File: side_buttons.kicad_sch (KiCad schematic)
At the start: 1 part, among them J4 Conn_01x08

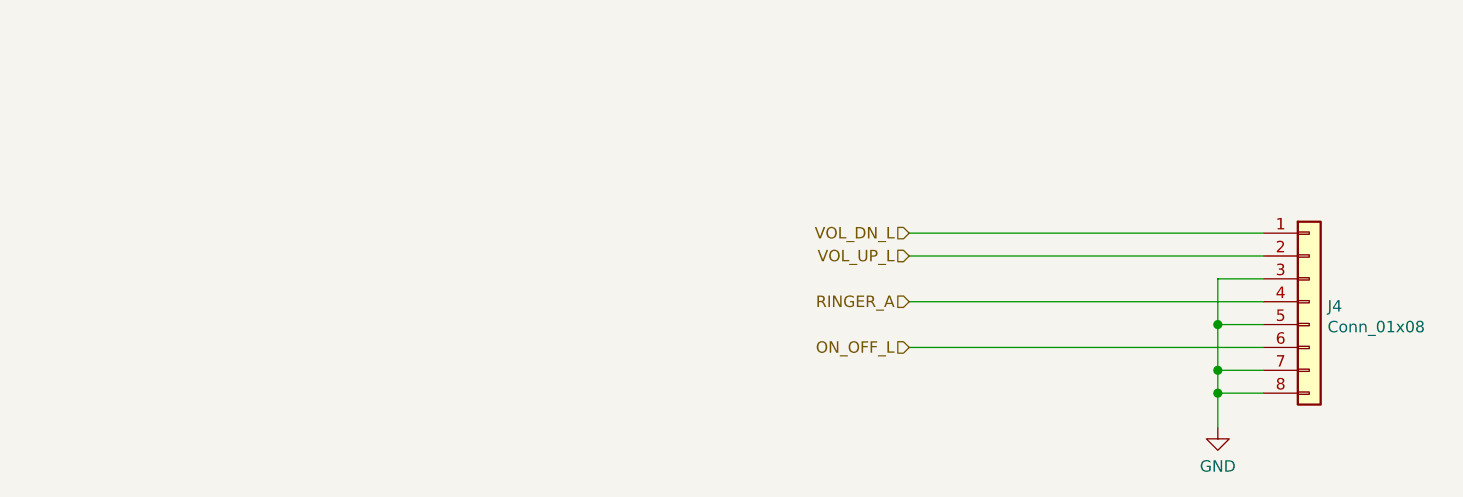
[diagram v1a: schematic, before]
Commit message: Final touches on Radxa CM3 version of the board
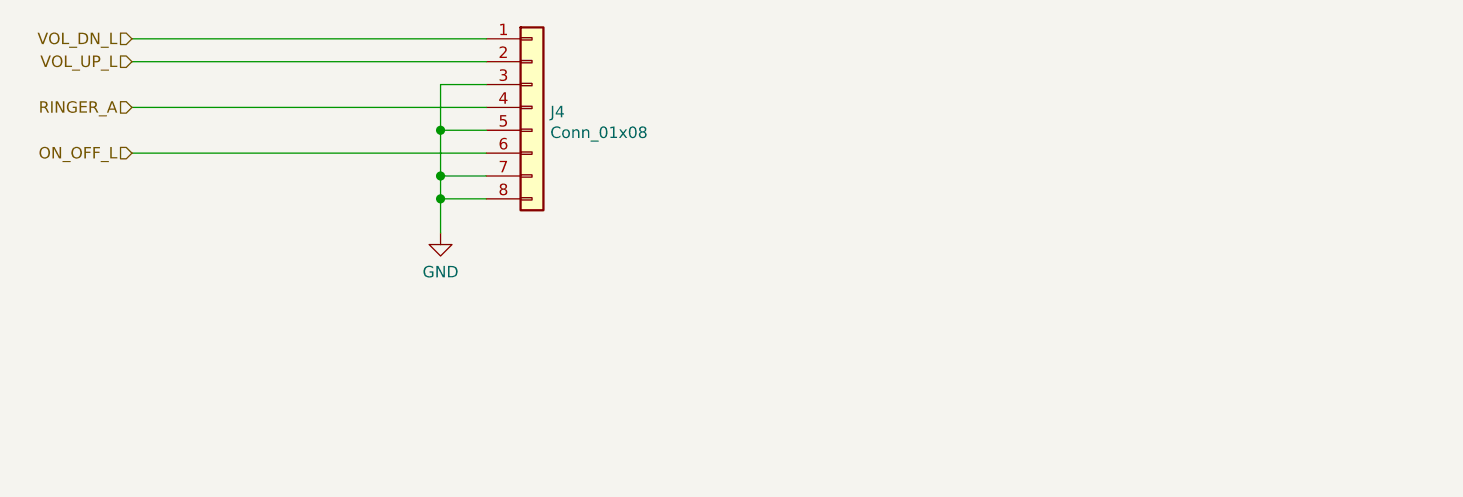
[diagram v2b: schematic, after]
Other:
- moved on the sheet: J4
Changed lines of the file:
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@@
 (kicad_sch (version 20211123) (generator eeschema)
-  (paper "A4")
-  (junction (at 213.36 86.36) (diameter 1.016) (color 0 0 0 0)
+  (paper "A5")
+  (junction (at 127 64.77) (diameter 1.016) (color 0 0 0 0)
   )
-  (junction (at 213.36 93.98) (diameter 1.016) (color 0 0 0 0)
+  (junction (at 127 72.39) (diameter 1.016) (color 0 0 0 0)
   )
-  (junction (at 213.36 91.44) (diameter 1.016) (color 0 0 0 0)
+  (junction (at 127 69.85) (diameter 1.016) (color 0 0 0 0)
   )
-  (wire (pts (xy 179.07 76.2) (xy 218.44 76.2))
+  (wire (pts (xy 92.71 54.61) (xy 132.08 54.61))
     (stroke (width 0) (type solid) (color 0 0 0 0))
   )
-  (wire (pts (xy 213.36 81.28) (xy 213.36 86.36))
+  (wire (pts (xy 127 59.69) (xy 127 64.77))
     (stroke (width 0) (type solid) (color 0 0 0 0))
   )
-  (wire (pts (xy 213.36 86.36) (xy 213.36 91.44))
+  (wire (pts (xy 127 64.77) (xy 127 69.85))
     (stroke (width 0) (type solid) (color 0 0 0 0))
   )
-  (wire (pts (xy 213.36 91.44) (xy 213.36 93.98))
+  (wire (pts (xy 127 69.85) (xy 127 72.39))
     (stroke (width 0) (type solid) (color 0 0 0 0))
   )
-  (wire (pts (xy 213.36 93.98) (xy 213.36 97.79))
+  (wire (pts (xy 127 72.39) (xy 127 76.2))
     (stroke (width 0) (type solid) (color 0 0 0 0))
   )
-  (wire (pts (xy 218.44 81.28) (xy 213.36 81.28))
+  (wire (pts (xy 132.08 59.69) (xy 127 59.69))
     (stroke (width 0) (type solid) (color 0 0 0 0))
   )
-  (wire (pts (xy 213.36 86.36) (xy 218.44 86.36))
+  (wire (pts (xy 127 64.77) (xy 132.08 64.77))
     (stroke (width 0) (type solid) (color 0 0 0 0))
   )
-  (wire (pts (xy 179.07 88.9) (xy 218.44 88.9))
+  (wire (pts (xy 92.71 67.31) (xy 132.08 67.31))
     (stroke (width 0) (type solid) (color 0 0 0 0))
   )
-  (wire (pts (xy 213.36 93.98) (xy 218.44 93.98))
+  (wire (pts (xy 127 72.39) (xy 132.08 72.39))
     (stroke (width 0) (type solid) (color 0 0 0 0))
   )
-  (wire (pts (xy 179.07 78.74) (xy 218.44 78.74))
+  (wire (pts (xy 92.71 57.15) (xy 132.08 57.15))
     (stroke (width 0) (type solid) (color 0 0 0 0))
   )
-  (wire (pts (xy 213.36 91.44) (xy 218.44 91.44))
+  (wire (pts (xy 127 69.85) (xy 132.08 69.85))
     (stroke (width 0) (type solid) (color 0 0 0 0))
   )
-  (wire (pts (xy 179.07 83.82) (xy 218.44 83.82))
+  (wire (pts (xy 92.71 62.23) (xy 132.08 62.23))
     (stroke (width 0) (type solid) (color 0 0 0 0))
   )
-  (hierarchical_label "VOL_UP_L" (shape input) (at 179.07 78.74 180)
+  (hierarchical_label "VOL_UP_L" (shape input) (at 92.71 57.15 180)
     (effects (font (size 1.27 1.27)) (justify right))
   )
-  (hierarchical_label "ON_OFF_L" (shape input) (at 179.07 88.9 180)
+  (hierarchical_label "ON_OFF_L" (shape input) (at 92.71 67.31 180)
     (effects (font (size 1.27 1.27)) (justify right))
   )
-  (hierarchical_label "VOL_DN_L" (shape input) (at 179.07 76.2 180)
+  (hierarchical_label "VOL_DN_L" (shape input) (at 92.71 54.61 180)
     (effects (font (size 1.27 1.27)) (justify right))
   )
-  (hierarchical_label "RINGER_A" (shape input) (at 179.07 83.82 180)
+  (hierarchical_label "RINGER_A" (shape input) (at 92.71 62.23 180)
     (effects (font (size 1.27 1.27)) (justify right))
   )
-  (symbol (lib_id "power:GND") (at 213.36 97.79 0) (unit 1)
+  (symbol (lib_id "power:GND") (at 127 76.2 0) (unit 1)
     (in_bom yes) (on_board yes) (fields_autoplaced)
-    (property "Reference" "#PWR0144" (id 0) (at 213.36 104.14 0)
+    (property "Reference" "#PWR0144" (id 0) (at 127 82.55 0)
       (effects (font (size 1.27 1.27)) hide)
     )
-    (property "Value" "GND" (id 1) (at 213.36 102.1144 0))
-    (property "Footprint" "" (id 2) (at 213.36 97.79 0)
+    (property "Value" "GND" (id 1) (at 127 80.5244 0))
+    (property "Footprint" "" (id 2) (at 127 76.2 0)
       (effects (font (size 1.27 1.27)) hide)
     )
-    (property "Datasheet" "" (id 3) (at 213.36 97.79 0)
+    (property "Datasheet" "" (id 3) (at 127 76.2 0)
       (effects (font (size 1.27 1.27)) hide)
     )
     (pin "1")
   )
-  (symbol (lib_id "Connector_Generic:Conn_01x08") (at 223.52 83.82 0) (unit 1)
+  (symbol (lib_id "Connector_Generic:Conn_01x08") (at 137.16 62.23 0) (unit 1)
     (in_bom yes) (on_board yes) (fields_autoplaced)
-    (property "Reference" "J4" (id 0) (at 225.5521 84.3291 0)
+    (property "Reference" "J4" (id 0) (at 139.1921 62.7391 0)
       (effects (font (size 1.27 1.27)) (justify left))
     )
-    (property "Value" "Conn_01x08" (id 1) (at 225.5521 86.6278 0)
+    (property "Value" "Conn_01x08" (id 1) (at 139.1921 65.0378 0)
       (effects (font (size 1.27 1.27)) (justify left))
     )
-    (property "Footprint" "footprints:78171-0006" (id 2) (at 223.52 83.82 0)
+    (property "Footprint" "footprints:78171-0006" (id 2) (at 137.16 62.23 0)
       (effects (font (size 1.27 1.27)) hide)
     )
-    (property "Datasheet" "~" (id 3) (at 223.52 83.82 0)
+    (property "Datasheet" "~" (id 3) (at 137.16 62.23 0)
       (effects (font (size 1.27 1.27)) hide)
     )
